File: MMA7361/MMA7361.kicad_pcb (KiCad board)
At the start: 2 copper layers, 22.4 x 20.3 mm, 16 parts, among them J1 Conn_01x05, J2 Conn_01x05, U1 RT9161, U2 MMA7361L

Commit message: The last version have been added
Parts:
- U2: footprint MMA7260Q:QFN-16 -> qfn-16:QFN-16
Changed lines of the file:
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@@
-(kicad_pcb (version 20171130) (host pcbnew "(5.0.0)")
+(kicad_pcb (version 20171130) (host pcbnew "(5.0.1)-4")
   (general
     (thickness 1.6)
-    (drawings 11)
+    (drawings 13)
     (tracks 86)
     (zones 0)
@@
     (add_net VCC)
   )
+  (module qfn-16:QFN-16 (layer F.Cu)
+    (at 153.162 91.694)
+    (descr "16 LEAD QFN CASE 1622-01<br>E.g. MMA7260Q")
+    (attr smd)
+    (fp_text reference U2 (at -3.81 0) (layer F.SilkS)
+      (effects (font (size 0.801591 0.801591) (thickness 0.05)))
+    )
+    (fp_text value MMA7361L (at -0.2 -3.8) (layer F.Fab)
+      (effects (font (size 0.800764 0.800764) (thickness 0.05)))
+    )
+    (fp_circle (center -3.7 3.5) (end -3.2877 3.5) (layer F.SilkS) (width 0.1))
+    (fp_line (start 3 3) (end 3 2.5) (layer F.SilkS) (width 0.127))
+    (fp_line (start 2.5 3) (end 3 3) (layer F.SilkS) (width 0.127))
+    (fp_line (start -3 3) (end -2.5 3) (layer F.SilkS) (width 0.127))
+    (fp_line (start -3 2.5) (end -3 3) (layer F.SilkS) (width 0.127))
+    (fp_line (start 3 -3) (end 3 -2.5) (layer F.SilkS) (width 0.127))
+    (fp_line (start 2.5 -3) (end 3 -3) (layer F.SilkS) (width 0.127))
+    (fp_line (start -3 -3) (end -3 -2.5) (layer F.SilkS) (width 0.127))
+    (fp_line (start -2.5 -3) (end -3 -3) (layer F.SilkS) (width 0.127))
+    (fp_line (start -3 3) (end -3 -3) (layer F.CrtYd) (width 0.127))
+    (fp_line (start 3 3) (end -3 3) (layer F.CrtYd) (width 0.127))
+    (fp_line (start 3 -3) (end 3 3) (layer F.CrtYd) (width 0.127))
+    (fp_line (start -3 -3) (end 3 -3) (layer F.CrtYd) (width 0.127))
+    (pad 16 smd rect (at -2.75 1.5 270) (size 0.5 0.55) (layers F.Cu F.Paste F.Mask))
+    (pad 15 smd rect (at -2.75 0.5 270) (size 0.5 0.55) (layers F.Cu F.Paste F.Mask))
+    (pad 14 smd rect (at -2.75 -0.5 270) (size 0.5 0.55) (layers F.Cu F.Paste F.Mask))
+    (pad 13 smd rect (at -2.75 -1.5 270) (size 0.5 0.55) (layers F.Cu F.Paste F.Mask)
+      (net 12 "/MMA 7361 Module/SelfTest"))
+    (pad 12 smd rect (at -1.5 -2.75 180) (size 0.5 0.55) (layers F.Cu F.Paste F.Mask)
+      (net 16 "Net-(U2-Pad12)"))
+    (pad 11 smd rect (at -0.5 -2.75 180) (size 0.5 0.55) (layers F.Cu F.Paste F.Mask)
+      (net 15 "Net-(U2-Pad11)"))
+    (pad 10 smd rect (at 0.5 -2.75 180) (size 0.5 0.55) (layers F.Cu F.Paste F.Mask)
+      (net 5 "/MMA 7361 Module/g-Select"))
+    (pad 9 smd rect (at 1.5 -2.75 180) (size 0.5 0.55) (layers F.Cu F.Paste F.Mask)
+      (net 4 "/MMA 7361 Module/Og-Detect"))
+    (pad 8 smd rect (at 2.75 -1.5 90) (size 0.5 0.55) (layers F.Cu F.Paste F.Mask)
+      (net 14 "Net-(U2-Pad8)"))
+    (pad 7 smd rect (at 2.75 -0.5 90) (size 0.5 0.55) (layers F.Cu F.Paste F.Mask)
+      (net 6 "/MMA 7361 Module/Sleep"))
+    (pad 6 smd rect (at 2.75 0.5 90) (size 0.5 0.55) (layers F.Cu F.Paste F.Mask)
+      (net 11 VCC))
+    (pad 5 smd rect (at 2.75 1.5 90) (size 0.5 0.55) (layers F.Cu F.Paste F.Mask)
+      (net 2 GND))
+    (pad 4 smd rect (at 1.5 2.75) (size 0.5 0.55) (layers F.Cu F.Paste F.Mask)
+      (net 8 "Net-(C1-Pad2)"))
+    (pad 3 smd rect (at 0.5 2.75) (size 0.5 0.55) (layers F.Cu F.Paste F.Mask)
+      (net 10 "Net-(C5-Pad2)"))
+    (pad 2 smd rect (at -0.5 2.75) (size 0.5 0.55) (layers F.Cu F.Paste F.Mask)
+      (net 9 "Net-(C3-Pad2)"))
+    (pad 1 smd rect (at -1.5 2.75) (size 0.5 0.55) (layers F.Cu F.Paste F.Mask)
+      (net 13 "Net-(U2-Pad1)"))
+    (pad P1 smd rect (at 0 0) (size 4.25 4.25) (layers F.Cu F.Paste F.Mask))
+  )
   (module Fiducial:Fiducial_0.5mm_Dia_1mm_Outer (layer F.Cu)
     (at 144 81)
@@
     (pad ~ smd circle (at 0 0) (size 0.5 0.5) (layers F.Cu F.Mask)
       (solder_mask_margin 0.25) (clearance 0.25))
-  )
-  (module MMA7260Q:QFN-16 (layer F.Cu)
-    (at 153.162 91.694)
-    (descr "16 LEAD QFN CASE 1622-01<br>E.g. MMA7260Q")
-    (attr smd)
-    (fp_text reference U2 (at -3.81 0) (layer F.SilkS)
-      (effects (font (size 0.801591 0.801591) (thickness 0.05)))
-    )
-    (fp_text value MMA7361L (at -0.2 -3.8) (layer F.Fab)
-      (effects (font (size 0.800764 0.800764) (thickness 0.05)))
-    )
-    (fp_line (start -3 -3) (end 3 -3) (layer Dwgs.User) (width 0.127))
-    (fp_line (start 3 -3) (end 3 3) (layer Dwgs.User) (width 0.127))
-    (fp_line (start 3 3) (end -3 3) (layer Dwgs.User) (width 0.127))
-    (fp_line (start -3 3) (end -3 -3) (layer Dwgs.User) (width 0.127))
-    (fp_line (start -2.5 -3) (end -3 -3) (layer F.SilkS) (width 0.127))
-    (fp_line (start -3 -3) (end -3 -2.5) (layer F.SilkS) (width 0.127))
-    (fp_line (start 2.5 -3) (end 3 -3) (layer F.SilkS) (width 0.127))
-    (fp_line (start 3 -3) (end 3 -2.5) (layer F.SilkS) (width 0.127))
-    (fp_line (start -3 2.5) (end -3 3) (layer F.SilkS) (width 0.127))
-    (fp_line (start -3 3) (end -2.5 3) (layer F.SilkS) (width 0.127))
-    (fp_line (start 2.5 3) (end 3 3) (layer F.SilkS) (width 0.127))
-    (fp_line (start 3 3) (end 3 2.5) (layer F.SilkS) (width 0.127))
-    (fp_circle (center -3.7 3.5) (end -3.2877 3.5) (layer F.SilkS) (width 0.1))
-    (pad P1 smd rect (at 0 0) (size 4.25 4.25) (layers F.Cu F.Paste F.Mask))
-    (pad 1 smd rect (at -1.5 2.75) (size 0.5 0.55) (layers F.Cu F.Paste F.Mask)
-      (net 13 "Net-(U2-Pad1)"))
-    (pad 2 smd rect (at -0.5 2.75) (size 0.5 0.55) (layers F.Cu F.Paste F.Mask)
-      (net 9 "Net-(C3-Pad2)"))
-    (pad 3 smd rect (at 0.5 2.75) (size 0.5 0.55) (layers F.Cu F.Paste F.Mask)
-      (net 10 "Net-(C5-Pad2)"))
-    (pad 4 smd rect (at 1.5 2.75) (size 0.5 0.55) (layers F.Cu F.Paste F.Mask)
-      (net 8 "Net-(C1-Pad2)"))
-    (pad 5 smd rect (at 2.75 1.5 90) (size 0.5 0.55) (layers F.Cu F.Paste F.Mask)
-      (net 2 GND))
-    (pad 6 smd rect (at 2.75 0.5 90) (size 0.5 0.55) (layers F.Cu F.Paste F.Mask)
-      (net 11 VCC))
-    (pad 7 smd rect (at 2.75 -0.5 90) (size 0.5 0.55) (layers F.Cu F.Paste F.Mask)
-      (net 6 "/MMA 7361 Module/Sleep"))
-    (pad 8 smd rect (at 2.75 -1.5 90) (size 0.5 0.55) (layers F.Cu F.Paste F.Mask)
-      (net 14 "Net-(U2-Pad8)"))
-    (pad 9 smd rect (at 1.5 -2.75 180) (size 0.5 0.55) (layers F.Cu F.Paste F.Mask)
-      (net 4 "/MMA 7361 Module/Og-Detect"))
-    (pad 10 smd rect (at 0.5 -2.75 180) (size 0.5 0.55) (layers F.Cu F.Paste F.Mask)
-      (net 5 "/MMA 7361 Module/g-Select"))
-    (pad 11 smd rect (at -0.5 -2.75 180) (size 0.5 0.55) (layers F.Cu F.Paste F.Mask)
-      (net 15 "Net-(U2-Pad11)"))
-    (pad 12 smd rect (at -1.5 -2.75 180) (size 0.5 0.55) (layers F.Cu F.Paste F.Mask)
-      (net 16 "Net-(U2-Pad12)"))
-    (pad 13 smd rect (at -2.75 -1.5 270) (size 0.5 0.55) (layers F.Cu F.Paste F.Mask)
-      (net 12 "/MMA 7361 Module/SelfTest"))
-    (pad 14 smd rect (at -2.75 -0.5 270) (size 0.5 0.55) (layers F.Cu F.Paste F.Mask))
-    (pad 15 smd rect (at -2.75 0.5 270) (size 0.5 0.55) (layers F.Cu F.Paste F.Mask))
-    (pad 16 smd rect (at -2.75 1.5 270) (size 0.5 0.55) (layers F.Cu F.Paste F.Mask))
   )
   (module Connector_PinHeader_1.00mm:PinHeader_1x05_P1.00mm_Vertical (layer F.Cu)
@@
     )
   )
-  (gr_text "NOTA: P1 no fue posible hallar el modelo 3d" (at 187.93 98.29) (layer Dwgs.User)
+  (dimension 22.352 (width 0.3) (layer Dwgs.User)
+    (gr_text "22,352 mm" (at 153.602 105.96) (layer Dwgs.User)
+      (effects (font (size 1.5 1.5) (thickness 0.3)))
+    )
+    (feature1 (pts (xy 164.778 98.78) (xy 164.778 104.446421)))
+    (feature2 (pts (xy 142.426 98.78) (xy 142.426 104.446421)))
+    (crossbar (pts (xy 142.426 103.86) (xy 164.778 103.86)))
+    (arrow1a (pts (xy 164.778 103.86) (xy 163.651496 104.446421)))
+    (arrow1b (pts (xy 164.778 103.86) (xy 163.651496 103.273579)))
+    (arrow2a (pts (xy 142.426 103.86) (xy 143.552504 104.446421)))
+    (arrow2b (pts (xy 142.426 103.86) (xy 143.552504 103.273579)))
+  )
+  (dimension 20.32 (width 0.3) (layer Dwgs.User)
+    (gr_text "20,320 mm" (at 171.195999 88.62 270) (layer Dwgs.User)
+      (effects (font (size 1.5 1.5) (thickness 0.3)))
+    )
+    (feature1 (pts (xy 164.778 98.78) (xy 169.68242 98.78)))
+    (feature2 (pts (xy 164.778 78.46) (xy 169.68242 78.46)))
+    (crossbar (pts (xy 169.095999 78.46) (xy 169.095999 98.78)))
+    (arrow1a (pts (xy 169.095999 98.78) (xy 168.509578 97.653496)))
+    (arrow1b (pts (xy 169.095999 98.78) (xy 169.68242 97.653496)))
+    (arrow2a (pts (xy 169.095999 78.46) (xy 168.509578 79.586504)))
+    (arrow2b (pts (xy 169.095999 78.46) (xy 169.68242 79.586504)))
+  )
+  (gr_text "NOTA: P1 no fue posible hallar el modelo 3d" (at 194.75 98.018) (layer Dwgs.User)
     (effects (font (size 1 1) (thickness 0.2)))
   )
-  (gr_text "* Componente: MMA7361\n* Pista: 0.250 mm\n* Margen: 0.25 mm\n* Mínimo ancho pista: 0.2 mm\n* Mínimo tamaño vía: 0.4 mm\n* Minimum via diameter: 1 mm\n* Terminación: HASL" (at 186.51 82.3) (layer Dwgs.User)
+  (gr_text "* Componente: MMA7361\n* Pista: 0.250 mm\n* Margen: 0.25 mm\n* Mínimo ancho pista: 0.2 mm\n* Mínimo tamaño vía: 0.4 mm\n* Minimum via diameter: 1 mm\n* Terminación: HASL" (at 189.924 83.54) (layer Dwgs.User)
     (effects (font (size 1 1) (thickness 0.2)))
   )

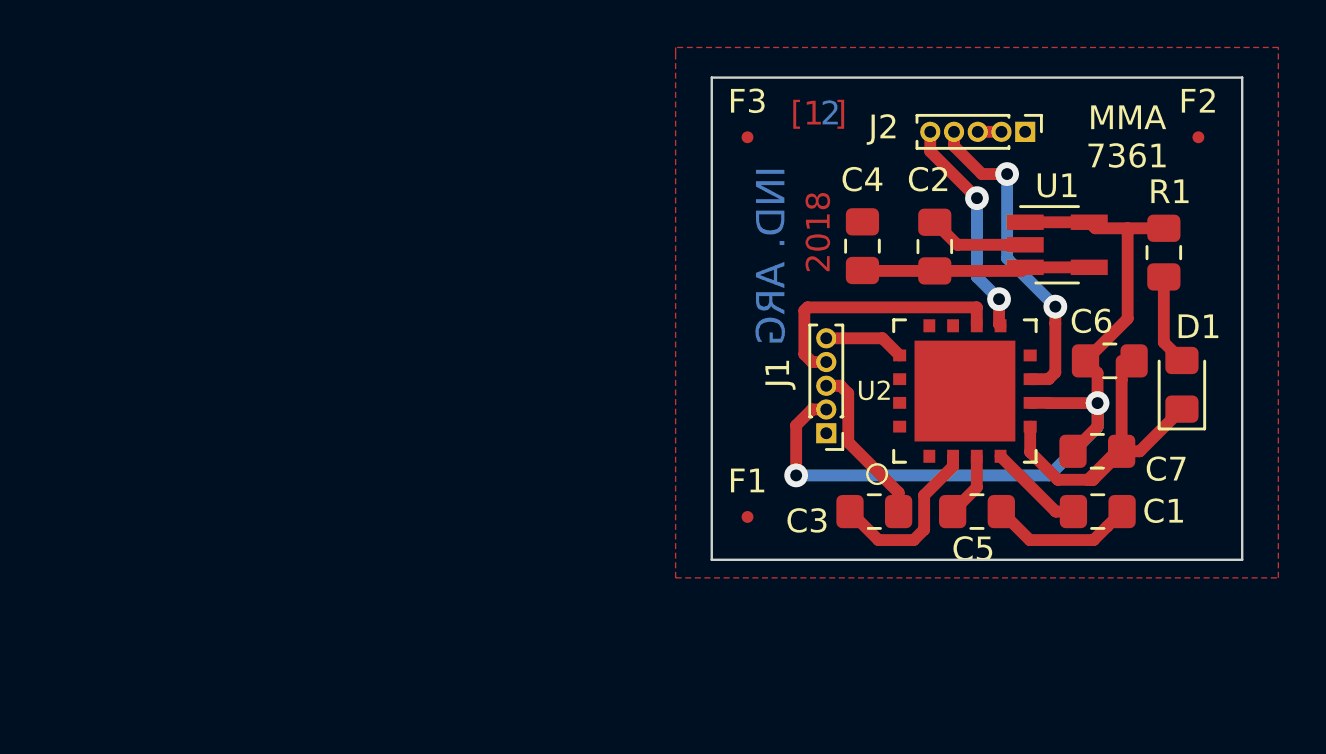
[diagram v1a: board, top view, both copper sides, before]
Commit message: The last version have been added
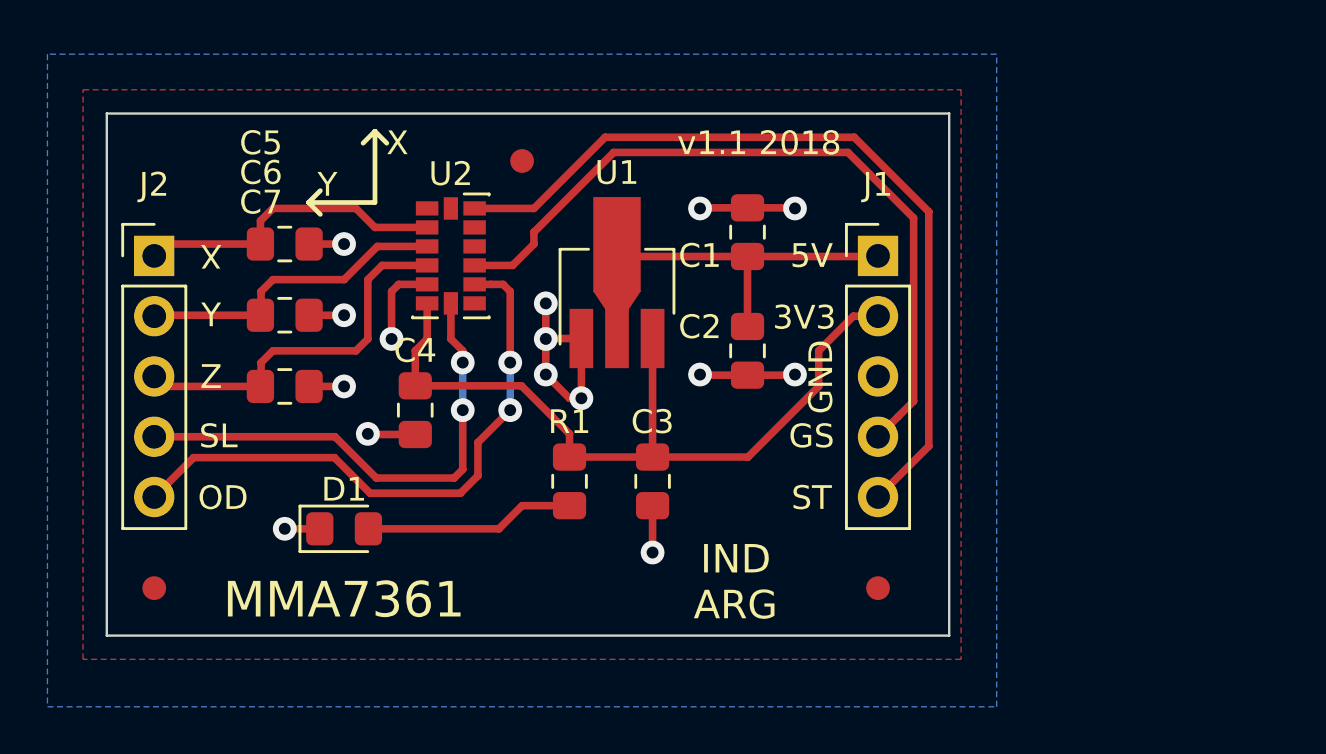
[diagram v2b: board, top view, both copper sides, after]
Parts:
- C1, C3: value 3.3nf -> 1 µF; footprint Capacitor_SMD:C_0805_2012Metric_Pad1.15x1.40mm_HandSolder -> Footprints:C_0805_2012Metric_Pad1.15x1.40mm_HandSolder
- C2: value 1 µF -> 470 µF; footprint Capacitor_SMD:C_0805_2012Metric_Pad1.15x1.40mm_HandSolder -> Footprints:C_0805_2012Metric_Pad1.15x1.40mm_HandSolder
- C4, C5: footprint Capacitor_SMD:C_0805_2012Metric_Pad1.15x1.40mm_HandSolder -> Footprints:C_0805_2012Metric_Pad1.15x1.40mm_HandSolder
- C6: value 1 µF -> 3.3nf; footprint Capacitor_SMD:C_0805_2012Metric_Pad1.15x1.40mm_HandSolder -> Footprints:C_0805_2012Metric_Pad1.15x1.40mm_HandSolder
- C7: value 470 µF -> 3.3nf; footprint Capacitor_SMD:C_0805_2012Metric_Pad1.15x1.40mm_HandSolder -> Footprints:C_0805_2012Metric_Pad1.15x1.40mm_HandSolder
- D1: footprint LED_SMD:LED_0805_2012Metric_Pad1.15x1.40mm_HandSolder -> Footprints:LED_0805_2012Metric_Pad1.15x1.40mm_HandSolder
- F1, F2, F3: footprint Fiducial:Fiducial_0.5mm_Dia_1mm_Outer -> Footprints:Fiducial_1mm_Dia_2mm_Outer
- J1, J2: footprint Connector_PinHeader_1.00mm:PinHeader_1x05_P1.00mm_Vertical -> Footprints:PinHeader_1x05_P2.54mm_Vertical
- R1: footprint Resistor_SMD:R_0805_2012Metric_Pad1.15x1.40mm_HandSolder -> Footprints:R_0805_2012Metric_Pad1.15x1.40mm_HandSolder
- U1: footprint Package_TO_SOT_SMD:SOT-23-5_HandSoldering -> Footprints:SOT-89-3_Handsoldering
- U2: footprint qfn-16:QFN-16 -> Footprints:LGA-14_3x5mm_P0.8mm_LayoutBorder1x6y
- moved F2 47.9 mm to (119.0, 100.0)
- moved J2 37.1 mm to (119.0, 86.0), turned to 0 degrees
- moved D1 35.8 mm to (127.0, 97.5), turned to 0 degrees
- moved C6 34.8 mm to (124.5, 88.5)
- moved C7 34.3 mm to (124.5, 91.5)
- moved C5 31.3 mm to (124.5, 85.5), turned to 0 degrees
- moved R1 26.8 mm to (136.5, 95.5)
- moved U2 22.4 mm to (131.5, 86.0)
- moved C4 20.1 mm to (130.0, 92.5), turned to 270 degrees
- moved F3 19.8 mm to (149.5, 100.0)
- moved C1 18.9 mm to (144.0, 85.0), turned to 90 degrees
- moved U1 18.7 mm to (138.5, 87.5), turned to 90 degrees
- moved F1 17.8 mm to (134.5, 82.0)
- moved C3 9.43 mm to (140.0, 95.5), turned to 270 degrees
- moved C2 9.03 mm to (144.0, 90.0), turned to 270 degrees
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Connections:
- net /MMA 7361 Module/Og-Detect renamed /Og-Detect
- net /MMA 7361 Module/SelfTest renamed /SelfTest
- net /MMA 7361 Module/Sleep renamed /~Sleep
- net /MMA 7361 Module/g-Select renamed /g-Select
- C1 pad 1: GND -> +5V
- C1 pad 2: Net-(C1-Pad2) -> GND
- C3 pad 1: GND -> VCC
- C3 pad 2: Net-(C3-Pad2) -> GND
- C4 pad 1: +5V -> VCC
- C5 pad 1: GND -> /X
- C5 pad 2: Net-(C5-Pad2) -> GND
- C6 pad 1: VCC -> /Y
- C7 pad 1: VCC -> /Z
- J1 pad 1: Net-(J1-Pad1) -> +5V
- J2 pad 1: GND -> /X
- J2 pad 2: GND -> /Y
- J2 pad 3: GND -> /Z
- U1 pad 1: VCC -> GND
- U1 pad 2: GND -> +5V
- U1 pad 3: +5V -> VCC
- U2 pad 14: (no net) -> Net-(U2-Pad14)
- U2 pad 2: Net-(C3-Pad2) -> /X
- U2 pad 3: Net-(C5-Pad2) -> /Y
- U2 pad 4: Net-(C1-Pad2) -> /Z
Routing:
- net /SelfTest: track 3.39 -> 34.6 mm
- net /g-Select: track 11.0 -> 31.7 mm
- net /Z: track 0.00 -> 15.8 mm
- net /Og-Detect: track 9.40 -> 25.2 mm
- net /Y: track 0.00 -> 13.3 mm
- net /X: track 0.00 -> 13.2 mm
- net +5V: track 9.63 -> 18.3 mm
- net Net-(C3-Pad2): track 7.40 -> 0.00 mm
- net /~Sleep: track 13.7 -> 21.1 mm
- net Net-(D1-Pad2): track 3.84 -> 8.88 mm
- net VCC: track 37.8 -> 33.3 mm, vias 2 -> 0
- net Net-(C1-Pad2): track 4.04 -> 0.00 mm
- net Net-(C5-Pad2): track 2.75 -> 0.00 mm
- net GND: track 33.2 -> 30.5 mm, vias 0 -> 15
- added copper zone on B.Cu, net GND
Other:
- board size 22.4 x 20.3 mm -> 35.5 x 22 mm
- net class Default: clearance 0.25 -> 0.2; trace_width 0.25 -> 0.32
- rule trace_clearance: 0.25 -> 0.2
- rule trace_min: 0.2 -> 0.32
- rule via_min_size: 0.4 -> 0.5
- board text added: "* Mínimos (Mayer 10 mils) * Componente: MMA7361 * Pista: 0.32 mm * Margen: 0.32 mm pista / 0.20 mm en pads LGA * Diametro vía: 1 mm * Agujero via: 0.5 mm * Material: FR-4 * Terminación: HASL"
- board text added: "3V3"
- board text added: "5V"
- board text added: "GND"
- board text added: "GS"
- board text added: "IND ARG"
- board text added: "MMA7361"
- board text added: "NOTA: U2 no fue posible hallar el modelo 3d, se adapto un BGA"
- board text added: "OD"
- board text added: "SL"
- board text added: "ST"
- board text added: "X"
- board text added: "Y"
- board text added: "Z"
- board text added: "v1.1 2018"
- board text removed: "* Componente: MMA7361 * Pista: 0.250 mm * Margen: 0.25 mm * Mínimo ancho pista: 0.2 mm * Mínimo tamaño vía: 0.4 mm * Minimum via diameter: 1 mm * Terminación: HASL"
- board text removed: "2"
- board text removed: "2018"
- board text removed: "IND. ARG"
- board text removed: "MMA 7361"
- board text removed: "NOTA: P1 no fue posible hallar el modelo 3d"
- board text removed: "[1 ]"
